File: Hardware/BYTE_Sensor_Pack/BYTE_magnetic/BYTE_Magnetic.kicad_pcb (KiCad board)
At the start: 2 copper layers, 18 x 23 mm, 16 parts, among them J1 PCB, U1 SI7210-B-11-IM2, U2 DRV2605YZFR, U4 SI7210-B-12-IM2, U5 SI7210-B-13-IM2, U6 SI7210-B-14-IM2

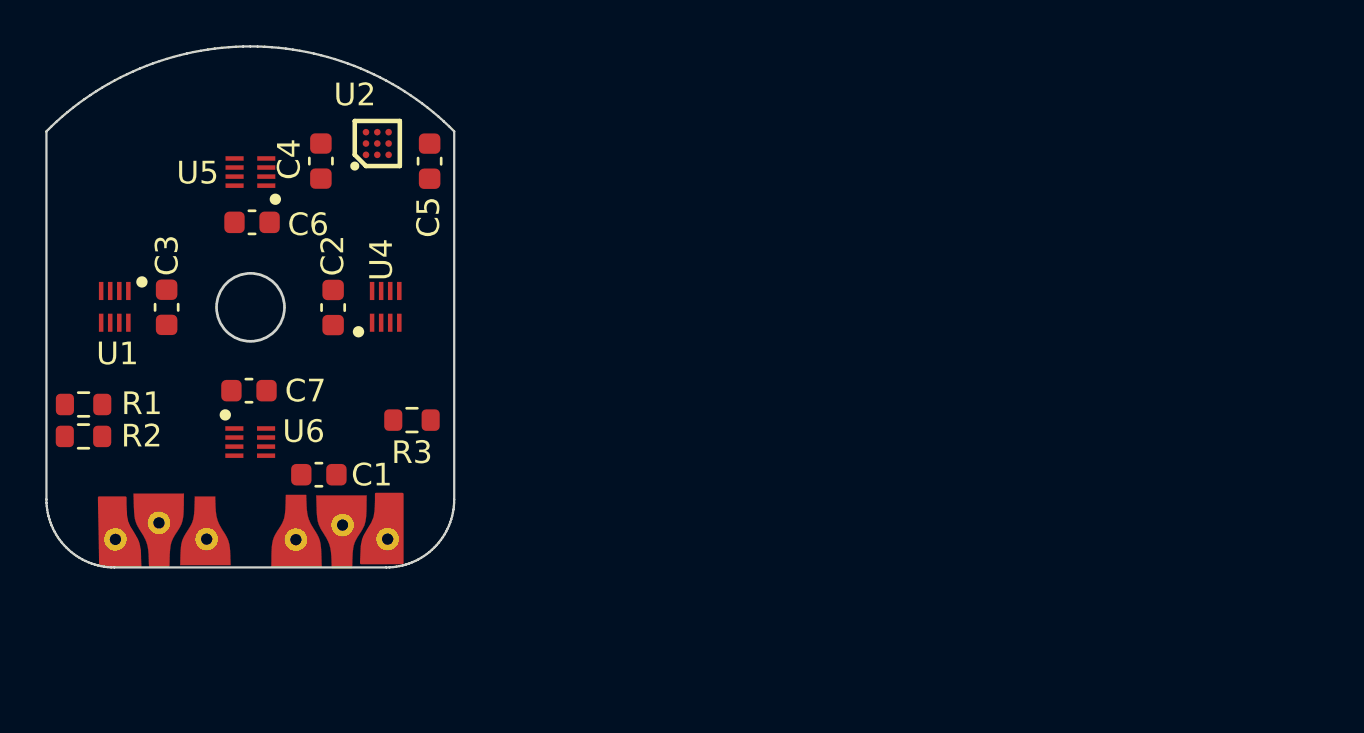
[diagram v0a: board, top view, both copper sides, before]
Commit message: update magnetic layout
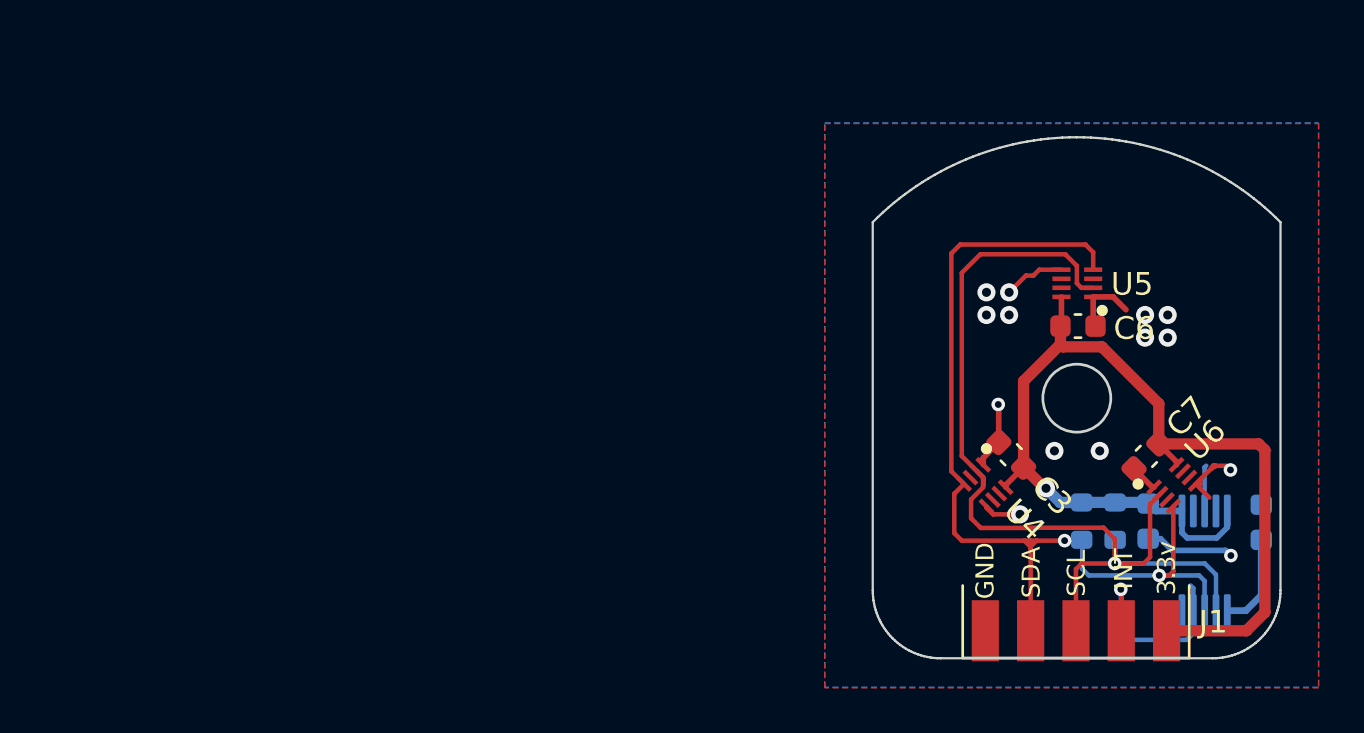
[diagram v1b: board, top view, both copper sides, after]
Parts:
- removed C1, C2: 0.1uF, Capacitor_SMD:C_0603_1608Metric
- removed the J1 at (146.4, 110.9)
- removed R3: 2.2K, Resistor_SMD:R_0603_1608Metric
- removed U2: DRV2605YZFR, BYTE_Sensors:BGA9C50P3X3_144X144X62
- added J1: Input, BYTE_Sensors:Flex_Connector, F.Cu at (181.9, 121.9)
- added J1: PCB, BYTE_Sensors:Senor_Only_PCB, F.Cu at (182.9, 114.9)
- added Ref**: Val**, BYTE_Sensors:Logo, F.Cu at (177.7, 92.4)
- C4, C5, R1, R2: moved to B.Cu
- U1: value SI7210-B-11-IM2 -> DRV2605LDGS; footprint BYTE_Sensors:SON40P140X160X40-8N-D -> Package_SO:VSSOP-10_3x3mm_P0.5mm; moved to B.Cu
- moved U1 49.4 mm to (187.6, 118.8), turned to 90 degrees
- moved R1 45.8 mm to (183.7, 117.1), turned to 270 degrees
- moved C4 44.5 mm to (190.1, 117.2), turned to 90 degrees
- moved R2 44.2 mm to (182.2, 117.1), turned to 270 degrees
- moved U6 40.9 mm to (186.3, 115.5), turned to 45 degrees
- moved C7 39.7 mm to (185.1, 114.2), turned to 225 degrees
- moved C3 37.8 mm to (179.1, 114.2), turned to 135 degrees
- moved U5 36.8 mm to (182.0, 106.6)
- moved C6 36.7 mm to (182.0, 108.5)
- moved C5 35.5 mm to (185.1, 117.1)
- moved U4 27.6 mm to (177.9, 115.5), turned to 315 degrees
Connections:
- C4 pad 1: /REG -> Net-(C4-Pad1)
- U1 pad 1: GND -> Net-(C4-Pad1)
- U1 pad 3: Net-(U1-Pad3) -> /SDA
- U1 pad 4: /SDA -> /IN_TRIG
- U1 pad 5: GND -> /EN
- U1 pad 6: Net-(U1-Pad6) -> +3V3
- U1 pad 7: Net-(U1-Pad3) -> Net-(M1-Pad1)
- U1 pad 8: +3V3 -> GND
- U4 pad 3: Net-(U4-Pad3) -> (no net)
- U4 pad 7: Net-(U4-Pad3) -> Net-(U4-Pad7)
- U5 pad 3: Net-(U5-Pad3) -> (no net)
- U5 pad 7: Net-(U5-Pad3) -> Net-(U5-Pad7)
- U6 pad 3: Net-(U6-Pad3) -> (no net)
- U6 pad 7: Net-(U6-Pad3) -> Net-(U6-Pad7)
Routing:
- net +3V3: track 0.00 -> 46.3 mm, vias 0 -> 1
- net /SCL: track 0.00 -> 43.7 mm, vias 0 -> 1
- net /SDA: track 0.00 -> 42.5 mm, vias 0 -> 2
- net GND: track 0.00 -> 20.6 mm, vias 0 -> 14
- net /IN_TRIG: track 0.00 -> 11.1 mm, vias 0 -> 1
- net Net-(C4-Pad1): track 0.00 -> 4.23 mm
- added copper zone on B.Cu, net GND
- added copper zone on F.Cu, net GND
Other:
- board text added: "3.3v"
- board text added: "GND"
- board text added: "INT"
- board text added: "SCL"
- board text added: "SDA"
